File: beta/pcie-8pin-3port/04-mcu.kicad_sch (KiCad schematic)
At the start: 9 parts, among them SW1 BOOT, SW2 RESET, U1 ESP32-C6-MINI-1-N4

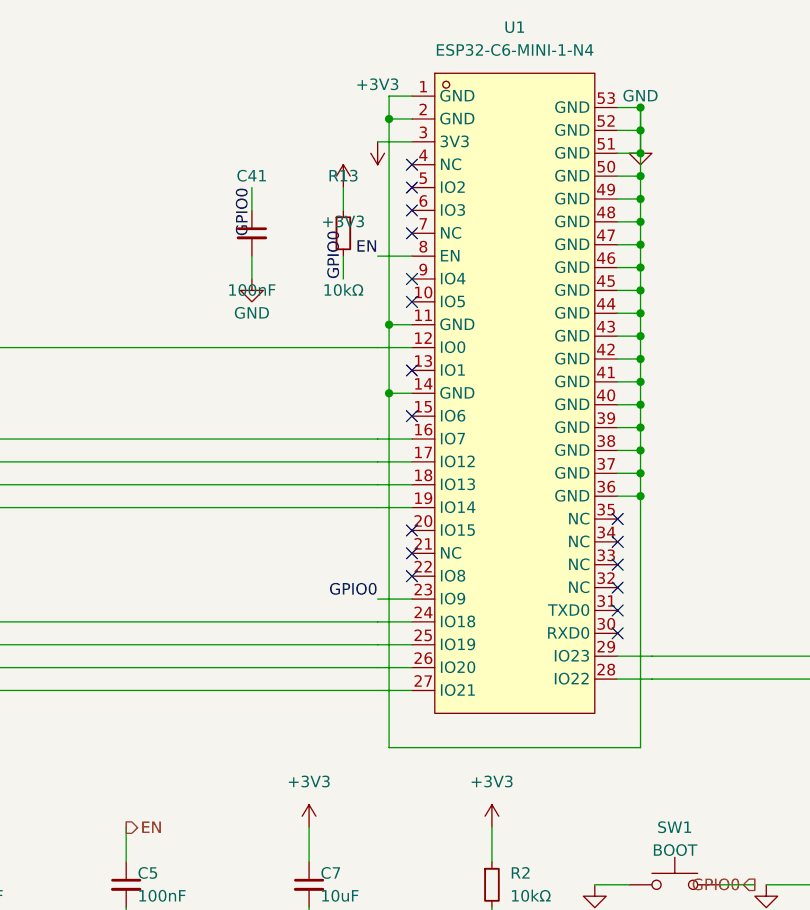
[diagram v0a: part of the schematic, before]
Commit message: Audit BETA electrical and pour pipeline
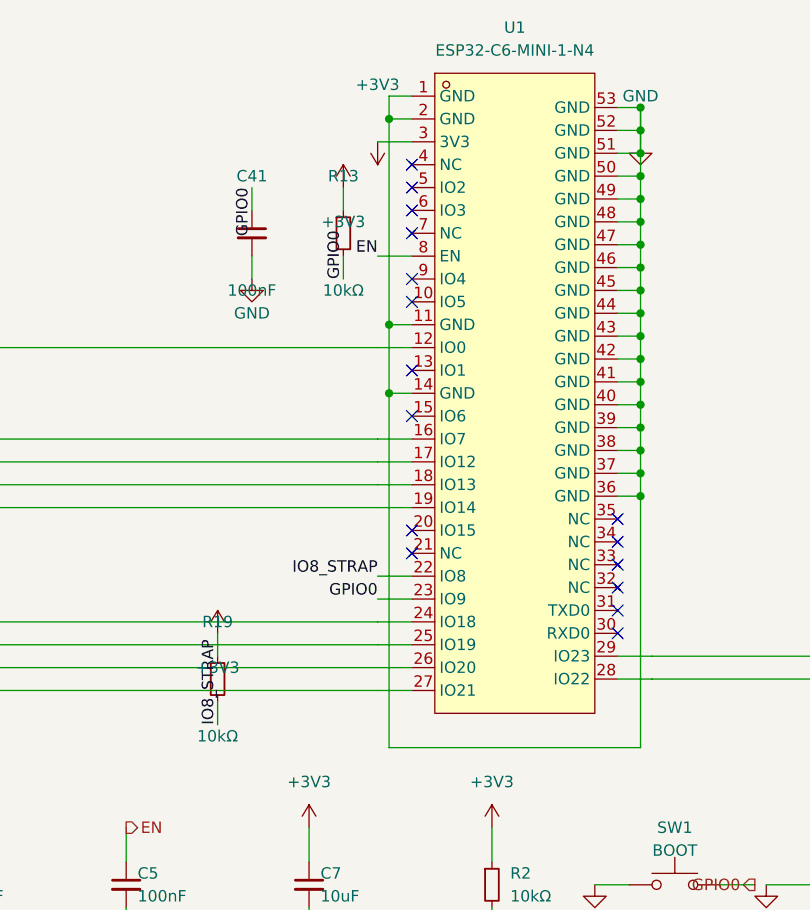
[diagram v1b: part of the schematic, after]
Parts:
- added R19: 10kΩ, cec-Resistor_SMD:R_0402_1005Metric, symbol cec-vendor:R_Small
- SW1, SW2: Manufacturer XKB -> XUNPU
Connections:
- net +3V3: now also R19.1
- net IO8_STRAP: now reaches U1.22 (IO8)
- net IO8_STRAP: now also R19.2
- no-connect marks 17 -> 16
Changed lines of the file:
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@@
 		(property "Value" "ESP32-C6-MINI-1-N4" (at 229.87 90.17 0) (effects (font (size 1.27 1.27))))
 		(property "Footprint" "cec-RF_Module:ESP32-C6-MINI-1" (at 229.87 128.27 0) (effects (font (size 1.27 1.27)) (hide yes)))
-		(property "Datasheet" "" (at 229.87 128.27 0) (effects (font (size 1.27 1.27)) (hide yes)))
+		(property "Datasheet" "https://documentation.espressif.com/esp32-c6-mini-1_mini-1u_datasheet_en.pdf" (at 229.87 128.27 0) (effects (font (size 1.27 1.27)) (hide yes)))
 		(property "Manufacturer" "Espressif Systems" (at 229.87 128.27 0) (effects (font (size 1.27 1.27)) (hide yes)))
 		(property "MPN" "ESP32-C6-MINI-1-N4" (at 229.87 128.27 0) (effects (font (size 1.27 1.27)) (hide yes)))
@@
 		(property "Value" "BOOT" (at 247.65 179.07 0) (effects (font (size 1.27 1.27))))
 		(property "Footprint" "cec-Button_Switch_SMD:TS-1088-AR02016" (at 247.65 182.88 0) (effects (font (size 1.27 1.27)) (hide yes)))
-		(property "Datasheet" "" (at 247.65 182.88 0) (effects (font (size 1.27 1.27)) (hide yes)))
-		(property "Manufacturer" "XKB" (at 247.65 182.88 0) (effects (font (size 1.27 1.27)) (hide yes)))
+		(property "Datasheet" "https://www.lcsc.com/datasheet/C720477.pdf" (at 247.65 182.88 0) (effects (font (size 1.27 1.27)) (hide yes)))
+		(property "Manufacturer" "XUNPU" (at 247.65 182.88 0) (effects (font (size 1.27 1.27)) (hide yes)))
 		(property "MPN" "TS-1088-AR02016" (at 247.65 182.88 0) (effects (font (size 1.27 1.27)) (hide yes)))
 		(property "LCSC" "C720477" (at 247.65 182.88 0) (effects (font (size 1.27 1.27)) (hide yes)))
@@
 		(property "Value" "RESET" (at 267.97 179.07 0) (effects (font (size 1.27 1.27))))
 		(property "Footprint" "cec-Button_Switch_SMD:TS-1088-AR02016" (at 267.97 182.88 0) (effects (font (size 1.27 1.27)) (hide yes)))
-		(property "Datasheet" "" (at 267.97 182.88 0) (effects (font (size 1.27 1.27)) (hide yes)))
-		(property "Manufacturer" "XKB" (at 267.97 182.88 0) (effects (font (size 1.27 1.27)) (hide yes)))
+		(property "Datasheet" "https://www.lcsc.com/datasheet/C720477.pdf" (at 267.97 182.88 0) (effects (font (size 1.27 1.27)) (hide yes)))
+		(property "Manufacturer" "XUNPU" (at 267.97 182.88 0) (effects (font (size 1.27 1.27)) (hide yes)))
 		(property "MPN" "TS-1088-AR02016" (at 267.97 182.88 0) (effects (font (size 1.27 1.27)) (hide yes)))
 		(property "LCSC" "C720477" (at 267.97 182.88 0) (effects (font (size 1.27 1.27)) (hide yes)))
@@
 	(no_connect (at 218.44 143.51))
 	(no_connect (at 218.44 146.05))
-	(no_connect (at 218.44 148.59))
-	(no_connect (at 241.3 154.94))
+		(no_connect (at 241.3 154.94))
 	(no_connect (at 241.3 152.4))
 	(no_connect (at 241.3 149.86))
@@
 		(stroke (width 0) (type default)))
 	(label "GPIO0" (at 210.82 115.57 270) (effects (font (size 1.27 1.27)) (justify left bottom)))
+	(wire (pts (xy 218.44 148.59) (xy 214.63 148.59))
+		(stroke (width 0) (type default)))
+	(label "IO8_STRAP" (at 214.63 148.59 180) (effects (font (size 1.27 1.27)) (justify right bottom)))
+	(symbol
+		(lib_id "cec-vendor:R_Small")
+		(at 196.85 160.02 0)
+		(unit 1)
+		(exclude_from_sim no)
+		(in_bom yes)
+		(on_board yes)
+		(dnp no)
+		(fields_autoplaced yes)
+		(property "Reference" "R19" (at 196.85 153.67 0) (effects (font (size 1.27 1.27))))
+		(property "Value" "10kΩ" (at 196.85 166.37 0) (effects (font (size 1.27 1.27))))
+		(property "Footprint" "cec-Resistor_SMD:R_0402_1005Metric" (at 196.85 160.02 0) (effects (font (size 1.27 1.27)) (hide yes)))
+		(property "Datasheet" "https://www.lcsc.com/product-detail/C25744.html" (at 196.85 160.02 0) (effects (font (size 1.27 1.27)) (hide yes)))
+		(property "Manufacturer" "UNI-ROYAL" (at 196.85 160.02 0) (effects (font (size 1.27 1.27)) (hide yes)))
+		(property "MPN" "0402WGF1002TCE" (at 196.85 160.02 0) (effects (font (size 1.27 1.27)) (hide yes)))
+		(property "LCSC" "C25744" (at 196.85 160.02 0) (effects (font (size 1.27 1.27)) (hide yes)))
+		(property "Description" "ESP32-C6 GPIO8 download-strap pull-up" (at 196.85 160.02 0) (effects (font (size 1.27 1.27)) (hide yes)))
+		(property "Note" "10 kohm follows Espressif ESP32-C6-DevKitC-1; GPIO8 must be high with GPIO9 low for joint download boot" (at 196.85 160.02 0) (effects (font (size 1.27 1.27)) (hide yes)))
+		(pin "1")
+		(pin "2")
+		(instances
+			(project "pcie8pin-3port-module"
+				(path "/a8ecf94e-f41a-4523-8cf1-1d72f47f3e7e/83ceb2d1-e50f-4838-831a-71136b7d1260" (reference "R19") (unit 1))
+			)
+		)
+	)
+	(wire (pts (xy 196.85 157.48) (xy 196.85 154.94))
+		(stroke (width 0) (type default)))
+	(symbol
+		(lib_id "cec-power:+3V3")
+		(at 196.85 154.94 0)
+		(unit 1)
+		(exclude_from_sim no)
+		(in_bom yes)
+		(on_board yes)
+		(dnp no)
+		(property "Reference" "#PWR0799" (at 196.85 152.4 0) (effects (font (size 1.27 1.27)) (hide yes)))
+		(property "Value" "+3V3" (at 196.85 158.75 0) (effects (font (size 1.27 1.27))))
+		(pin "1")
+		(instances
+			(project "pcie8pin-3port-module"
+				(path "/a8ecf94e-f41a-4523-8cf1-1d72f47f3e7e/83ceb2d1-e50f-4838-831a-71136b7d1260" (reference "#PWR0799") (unit 1))
+			)
+		)
+	)
+	(wire (pts (xy 196.85 162.56) (xy 196.85 165.1))
+		(stroke (width 0) (type default)))
+	(label "IO8_STRAP" (at 196.85 165.1 270) (effects (font (size 1.27 1.27)) (justify left bottom)))
 	(sheet_instances
 		(path "/83ceb2d1-e50f-4838-831a-71136b7d1260"
